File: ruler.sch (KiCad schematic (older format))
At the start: 83 parts, among them J1 USB_OTG, Q1 SOT23, Q2 SOT323, Q3 SOT883, Q4 SOT523, Q5 SOT223, Q6 SOT89, Q7 SuperSOT, SW1 KMR2, SW2 EVQPE1, SW3 B3U1000P, SW4 FSMCT, SW5 TL3315, SW6 FSM2JSM, SW7 JS202011SCQN, SW8 B3U, U1 QFN-0.5mm, U10 SOT963-6, U11 SSOP14, U12 SO16-L, U13 SOT666, U14 SOT1194, U15 SOT1333, U16 SOT669, U17 TSSOP 4.4x3mm, U18 SO4, U19 VSSOP, U2 LQFP, U3 SOIC, U4 BGA-0.8mm, U5 TSSOP 3x3mm, U6 MSOIC, U7 TSOP-0.95mm, U8 SOT23-6, U9 SOT23-8

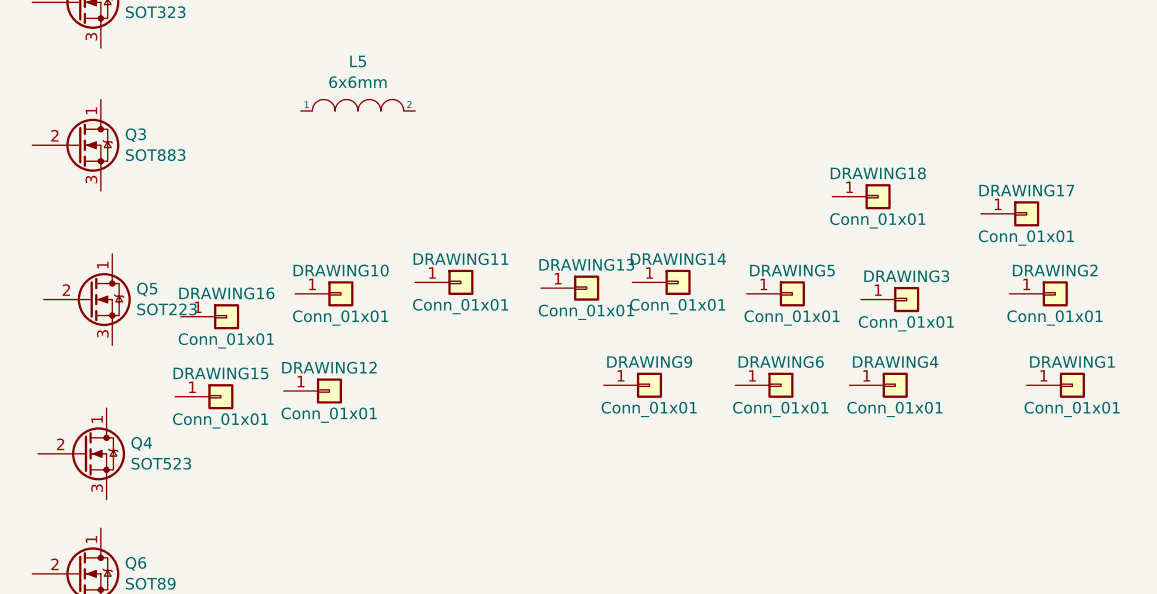
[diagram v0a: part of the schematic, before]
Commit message: Route
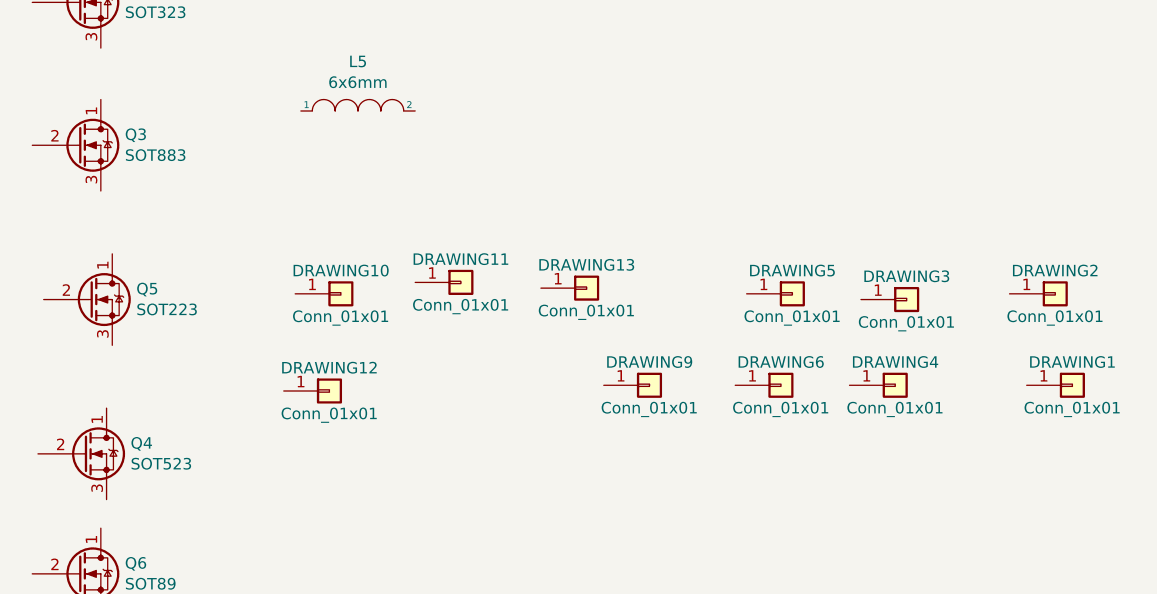
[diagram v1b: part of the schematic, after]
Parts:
- removed DRAWING14: Conn_01x01, drawings:mouse, symbol ruler-rescue:conn_Conn_01x01
- removed DRAWING15: Conn_01x01, drawings:chipmunk, symbol ruler-rescue:conn_Conn_01x01
- removed DRAWING16: Conn_01x01, drawings:weasel, symbol ruler-rescue:conn_Conn_01x01
- removed DRAWING17, DRAWING18: Conn_01x01, drawings:ant, symbol ruler-rescue:conn_Conn_01x01
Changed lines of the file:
@@
-$EndComp
-$Comp
-L ruler-rescue:conn_Conn_01x01 DRAWING14
-U 1 1 5AF42BAF
-P 9200 5750
-F 0 "DRAWING14" H 9200 5850 50  0000 C CNN
-F 1 "Conn_01x01" H 9200 5650 50  0000 C CNN
-F 2 "drawings:mouse" H 9200 5750 50  0001 C CNN
-F 3 "" H 9200 5750 50  0001 C CNN
-	1    9200 5750
-	1    0    0    -1
 $EndComp
 $Comp
@@
 $EndComp
 $Comp
-L ruler-rescue:conn_Conn_01x01 DRAWING15
-U 1 1 5B01E53E
-P 7200 6250
-F 0 "DRAWING15" H 7200 6350 50  0000 C CNN
-F 1 "Conn_01x01" H 7200 6150 50  0000 C CNN
-F 2 "drawings:chipmunk" H 7200 6250 50  0001 C CNN
-F 3 "" H 7200 6250 50  0001 C CNN
-	1    7200 6250
-	1    0    0    -1
-$EndComp
-$Comp
-L ruler-rescue:conn_Conn_01x01 DRAWING16
-U 1 1 5B01F029
-P 7225 5900
-F 0 "DRAWING16" H 7225 6000 50  0000 C CNN
-F 1 "Conn_01x01" H 7225 5800 50  0000 C CNN
-F 2 "drawings:weasel" H 7225 5900 50  0001 C CNN
-F 3 "" H 7225 5900 50  0001 C CNN
-	1    7225 5900
-	1    0    0    -1
-$EndComp
-$Comp
 L ruler-rescue:conn_Conn_01x01 U14
 U 1 1 5B01F626
@@
 	1    0    0    -1
 $EndComp
-$Comp
-L ruler-rescue:conn_Conn_01x01 DRAWING17
-U 1 1 5B026222
-P 10725 5450
-F 0 "DRAWING17" H 10725 5550 50  0000 C CNN
-F 1 "Conn_01x01" H 10725 5350 50  0000 C CNN
-F 2 "drawings:ant" H 10725 5450 50  0001 C CNN
-F 3 "" H 10725 5450 50  0001 C CNN
-	1    10725 5450
-	1    0    0    -1
-$EndComp
-$Comp
-L ruler-rescue:conn_Conn_01x01 DRAWING18
-U 1 1 5B0267EF
-P 10075 5375
-F 0 "DRAWING18" H 10075 5475 50  0000 C CNN
-F 1 "Conn_01x01" H 10075 5275 50  0000 C CNN
-F 2 "drawings:ant" H 10075 5375 50  0001 C CNN
-F 3 "" H 10075 5375 50  0001 C CNN
-	1    10075 5375
-	1    0    0    -1
-$EndComp

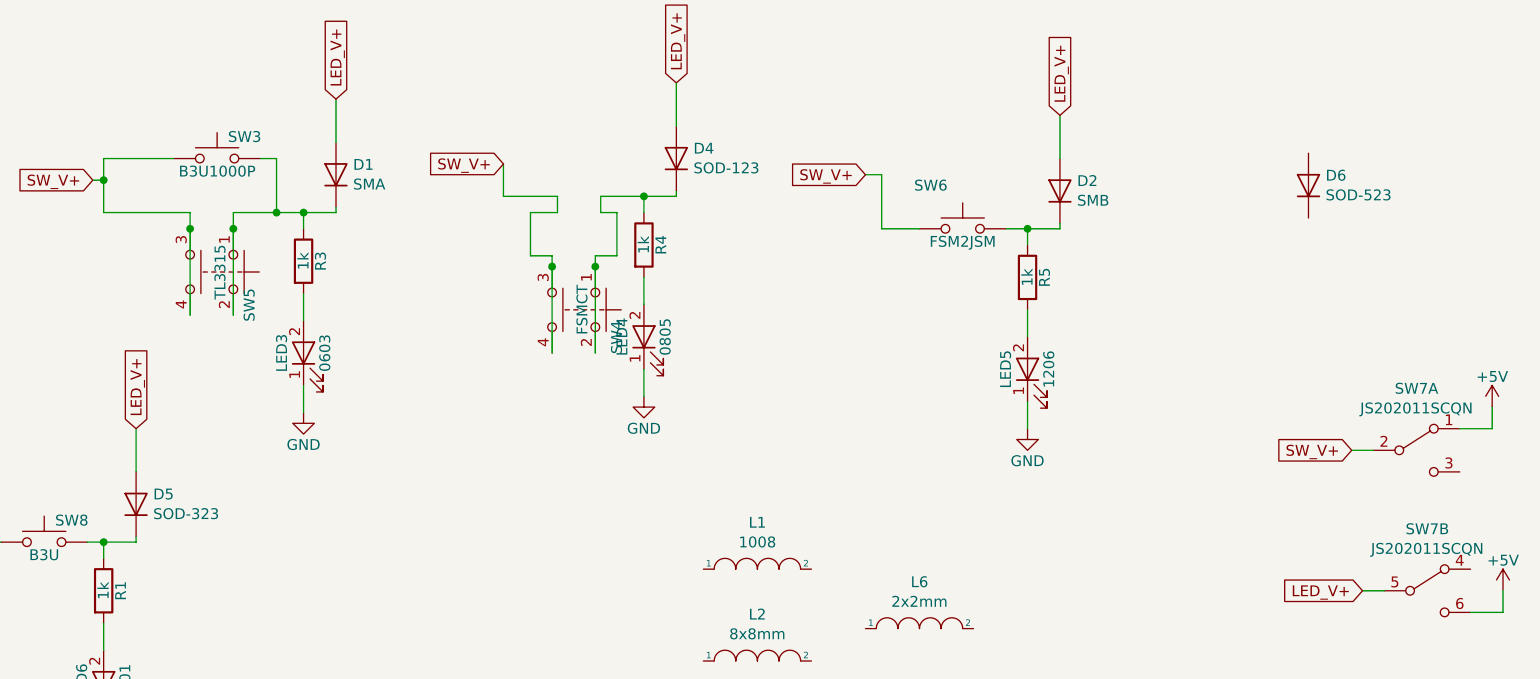
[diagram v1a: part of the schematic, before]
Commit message: Move some stuff around and plot
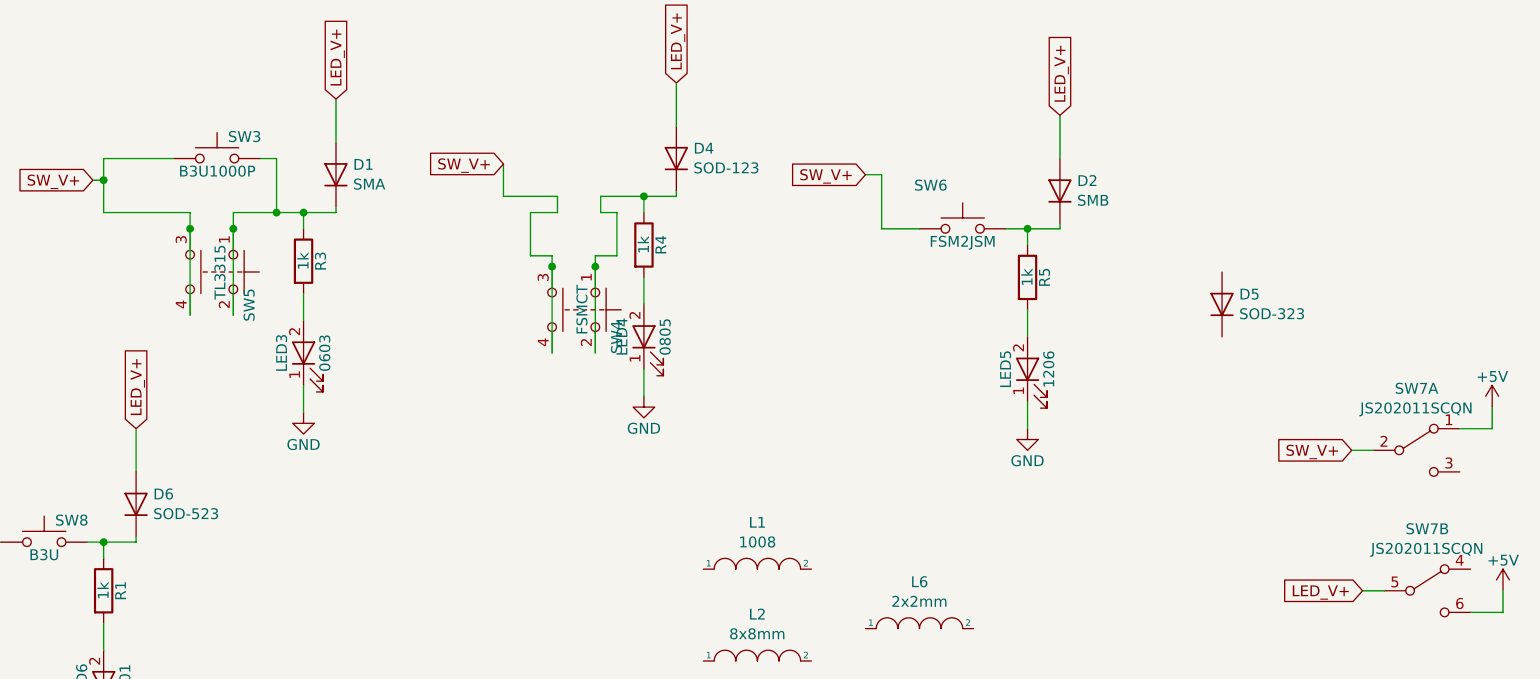
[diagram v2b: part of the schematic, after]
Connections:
- net LED_V+: now also D6.2 (A); no longer D5.2 (A)
- net at R1.1, SW8.2: now also D6.1 (K); no longer D5.1 (K)
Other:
- moved on the sheet: D5, D6
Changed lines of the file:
@@
 L ruler-rescue:device_D D5
 U 1 1 5AF4E276
-P 4800 2750
-F 0 "D5" V 4846 2671 50  0000 R CNN
-F 1 "SOD-323" V 4755 2671 50  0000 R CNN
-F 2 "KiCad/Diodes_SMD.pretty:D_SOD-323" H 4800 2750 50  0001 C CNN
-F 3 "" H 4800 2750 50  0001 C CNN
-	1    4800 2750
+P 9825 1825
+F 0 "D5" V 9871 1746 50  0000 R CNN
+F 1 "SOD-323" V 9780 1746 50  0000 R CNN
+F 2 "KiCad/Diodes_SMD.pretty:D_SOD-323" H 9825 1825 50  0001 C CNN
+F 3 "" H 9825 1825 50  0001 C CNN
+	1    9825 1825
 	0    -1   -1   0
 $EndComp
@@
 L ruler-rescue:device_D D6
 U 1 1 5AF4E2E0
-P 10225 1275
-F 0 "D6" V 10271 1196 50  0000 R CNN
-F 1 "SOD-523" V 10180 1196 50  0000 R CNN
-F 2 "KiCad/Diodes_SMD.pretty:D_SOD-523" H 10225 1275 50  0001 C CNN
-F 3 "" H 10225 1275 50  0001 C CNN
-	1    10225 1275
+P 4800 2750
+F 0 "D6" V 4846 2671 50  0000 R CNN
+F 1 "SOD-523" V 4755 2671 50  0000 R CNN
+F 2 "KiCad/Diodes_SMD.pretty:D_SOD-523" H 4800 2750 50  0001 C CNN
+F 3 "" H 4800 2750 50  0001 C CNN
+	1    4800 2750
 	0    -1   -1   0
 $EndComp
